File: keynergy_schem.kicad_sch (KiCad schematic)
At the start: 30 parts, among them J1 Conn_01x03_Pin, J2 Conn_01x03_Pin, J3 Conn_01x04_Pin, J4 Conn_01x03_Pin, J5 Conn_01x04_Pin, J6 Conn_01x03_Pin, J7 Conn_01x04_Pin, J8 Conn_01x03_Pin

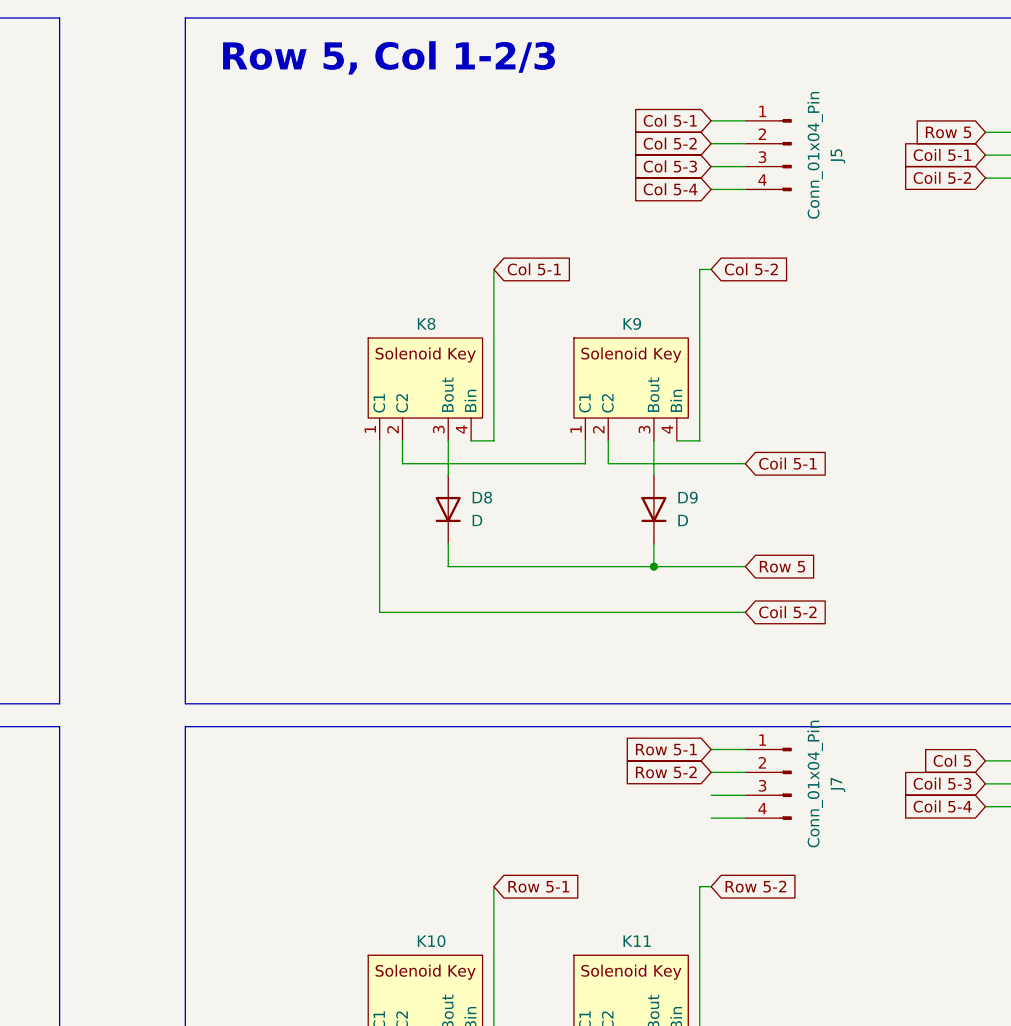
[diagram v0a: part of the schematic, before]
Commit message: new update
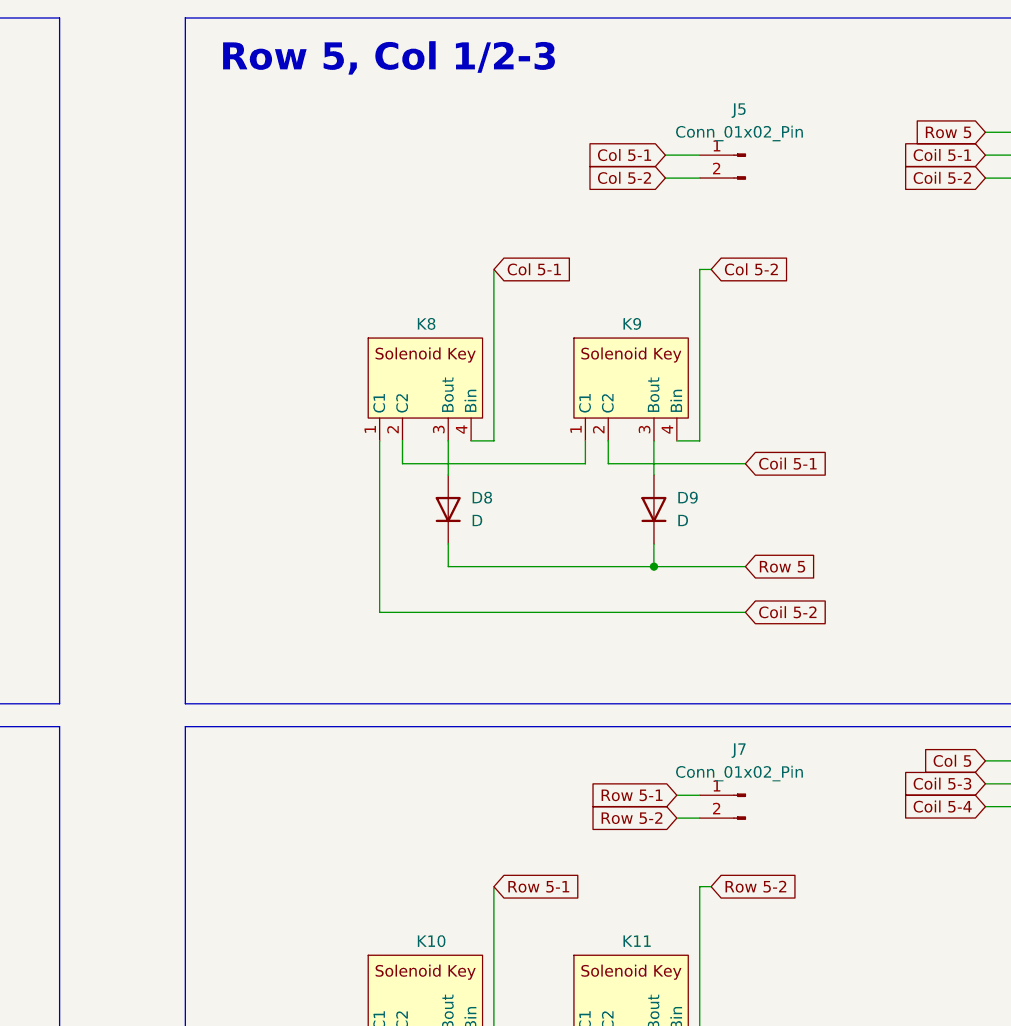
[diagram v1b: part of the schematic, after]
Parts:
- removed J5, J7: Conn_01x04_Pin, Connector_PinHeader_2.54mm:PinHeader_1x04_P2.54mm_Vertical, symbol Connector:Conn_01x04_Pin
- added J5, J7: Conn_01x02_Pin, Connector_PinHeader_2.54mm:PinHeader_1x02_P2.54mm_Vertical, symbol Connector:Conn_01x02_Pin
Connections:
- net Col 5-1: now also J5.1 (Pin_1)
- net Col 5-2: now also J5.2 (Pin_2)
- net Row 5-1: now also J7.1 (Pin_1)
- net Row 5-2: now also J7.2 (Pin_2)
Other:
- note added: "Row 5, Col 1/2-3"
- note removed: "Row 5, Col 1-2/3"
